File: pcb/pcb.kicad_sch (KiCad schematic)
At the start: 43 parts, among them J1 Conn_01x02_Socket, J2 Conn_01x04_Socket, U1 AP2112K-3.3TRG1, U2 W25Q16JVUXIQ, U3 RP2040, U4 DS4432U+T&amp;R, U5 AD8403ARUZ1-REEL, U6 ADG801BRTZ-REEL7, Y2 Crystal_GND24_Small

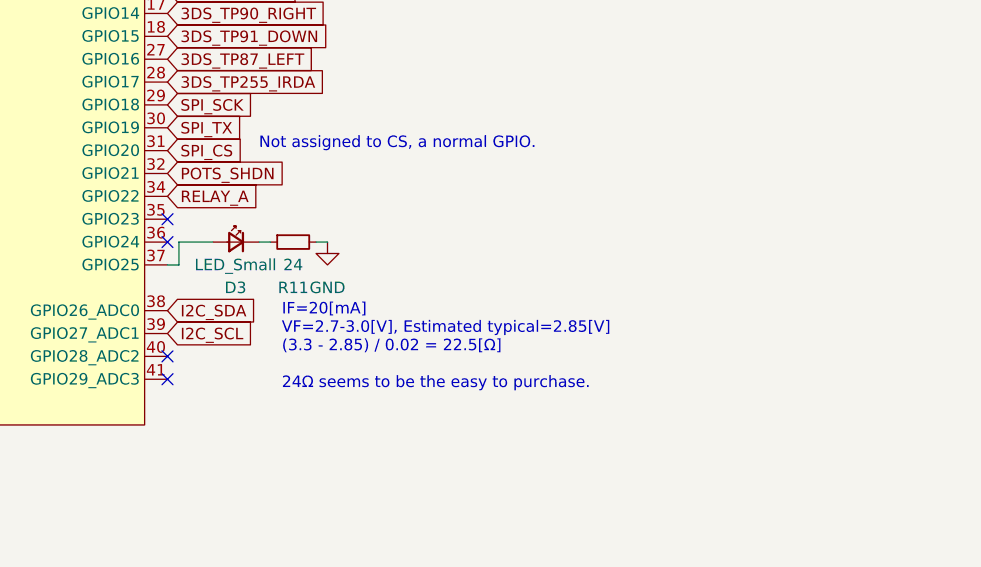
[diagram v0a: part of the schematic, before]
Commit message: Update schematic
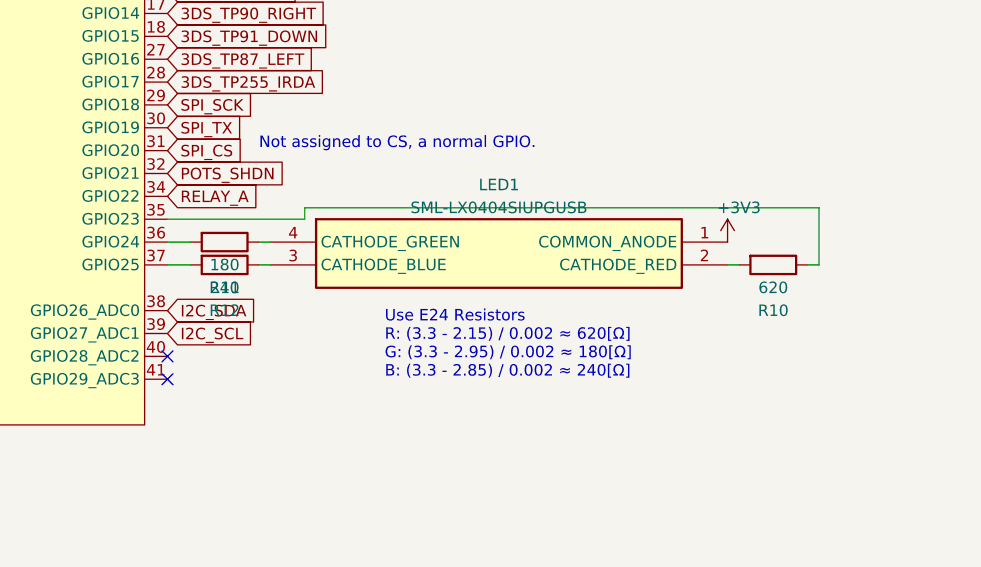
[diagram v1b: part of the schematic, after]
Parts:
- removed D3: LED_Small, LED_SMD:LED_0402_1005Metric, symbol Device:LED_Small
- removed R11: 24, Resistor_SMD:R_0402_1005Metric, symbol Device:R_Small
- added LED1: SML-LX0404SIUPGUSB, SML-LX0404SIUPGUSB, symbol SML-LX0404SIUPGUSB:SML-LX0404SIUPGUSB
- added R10: 620, Resistor_SMD:R_0402_1005Metric, symbol Device:R
- added R11: 180, Resistor_SMD:R_0402_1005Metric, symbol Device:R
- added R12: 240, Resistor_SMD:R_0402_1005Metric, symbol Device:R
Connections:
- net +3V3: now also LED1.1 (COMMON_ANODE)
- net at U3.35 (GPIO23): now also R10.1
- net at U3.36 (GPIO24): now also R11.2
- net at U3.37 (GPIO25): now also R12.2
- new net: LED1.2 (CATHODE_RED), R10.2
- new net: LED1.3 (CATHODE_BLUE), R12.1
- new net: LED1.4 (CATHODE_GREEN), R11.1
- no-connect marks 13 -> 11
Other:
- note added: "Use E24 Resistors R: (3.3 - 2.15) / 0.002 ≈ 620[Ω] G: (3.3 - 2.95) / 0.002 ≈ 180[Ω] B: (3.3 - 2.85) / 0.002 ≈ 240[Ω]"
- note removed: "IF=20[mA] VF=2.7-3.0[V], Estimated typical=2.85[V] (3.3 - 2.85) / 0.02 = 22.5[Ω] 24Ω seems to be the easy to purchase."

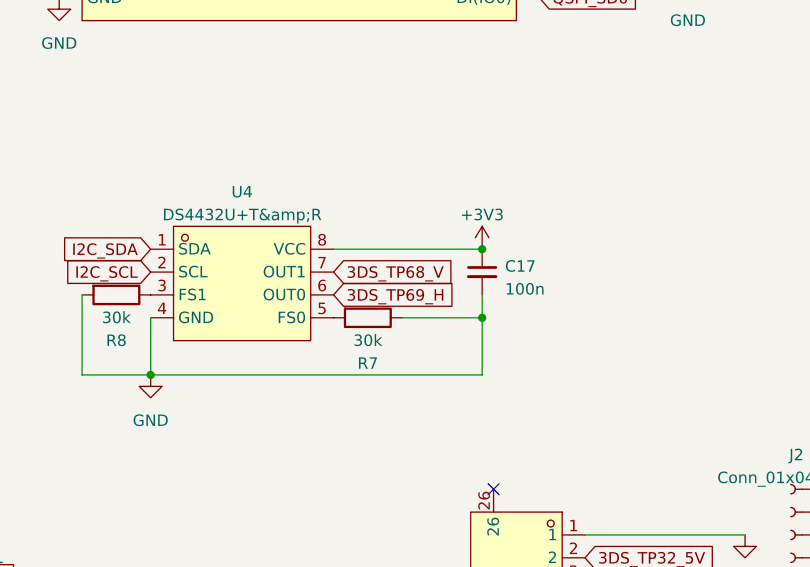
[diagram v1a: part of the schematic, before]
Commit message: Update PCB
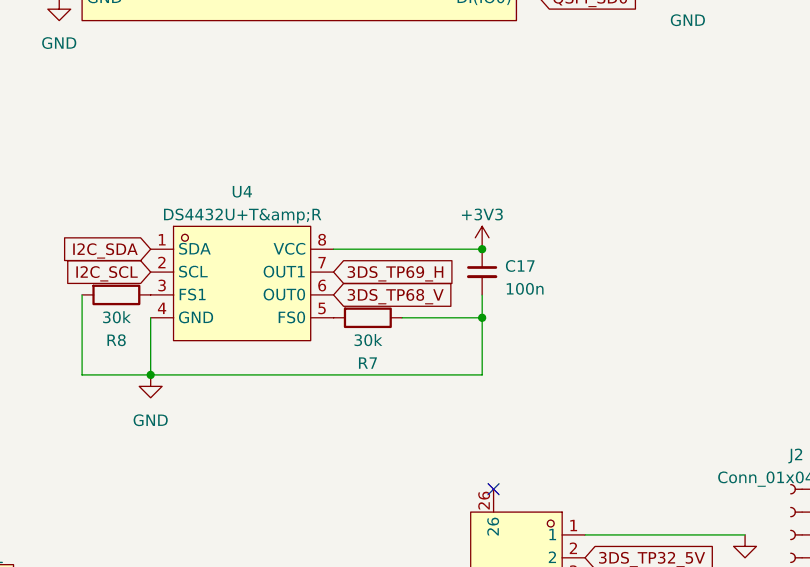
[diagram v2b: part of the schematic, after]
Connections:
- net 3DS_TP68_V: now also U4.6 (OUT0); no longer U4.7 (OUT1)
- net 3DS_TP69_H: now also U4.7 (OUT1); no longer U4.6 (OUT0)

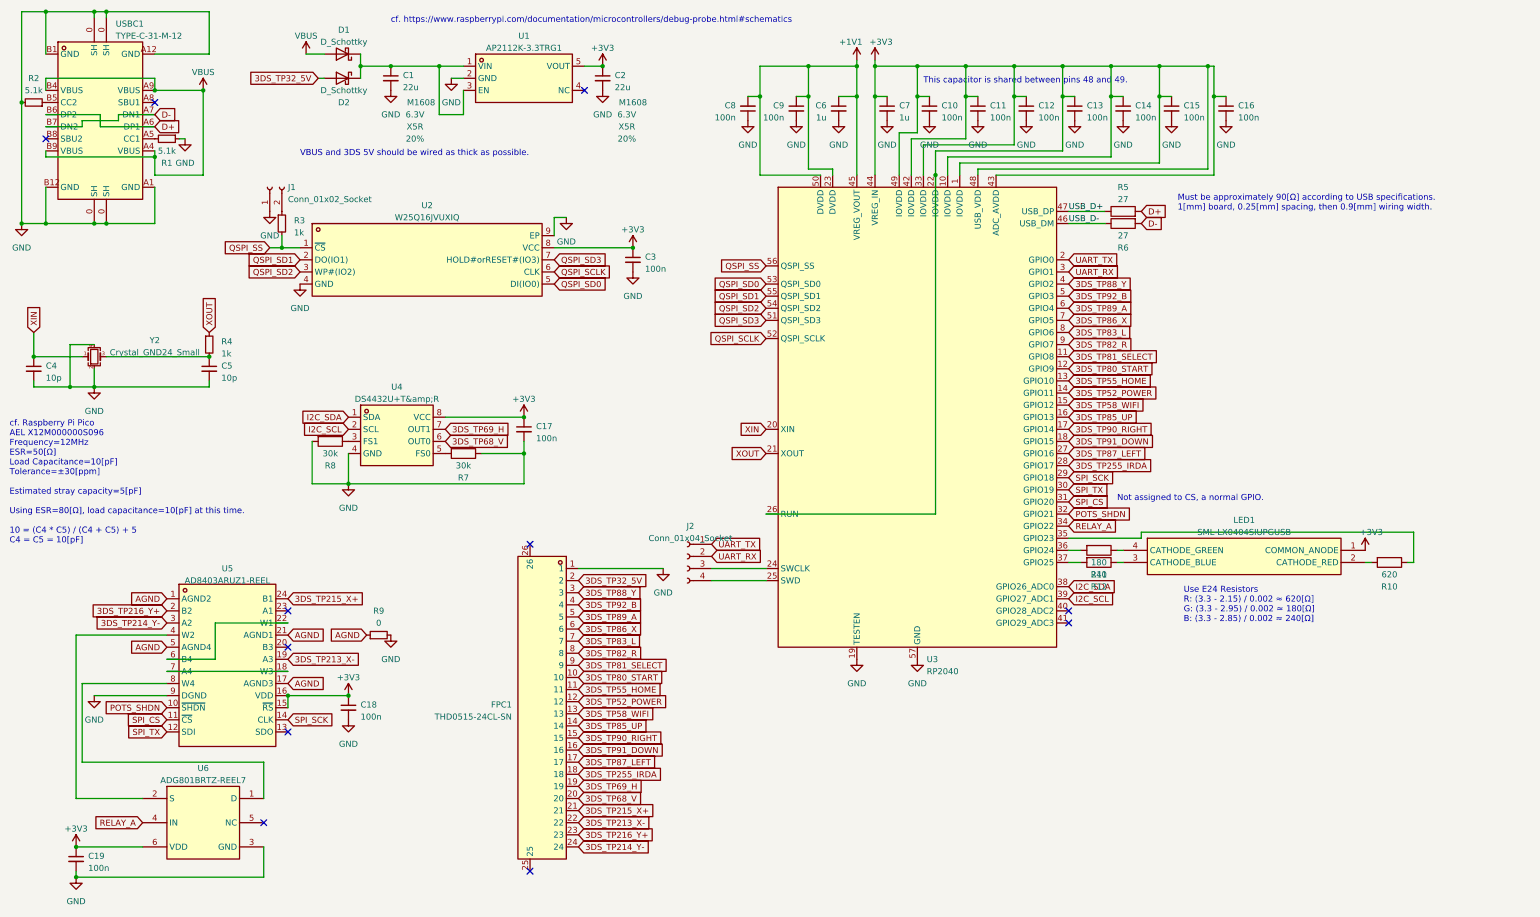
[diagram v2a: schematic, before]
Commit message: Resize
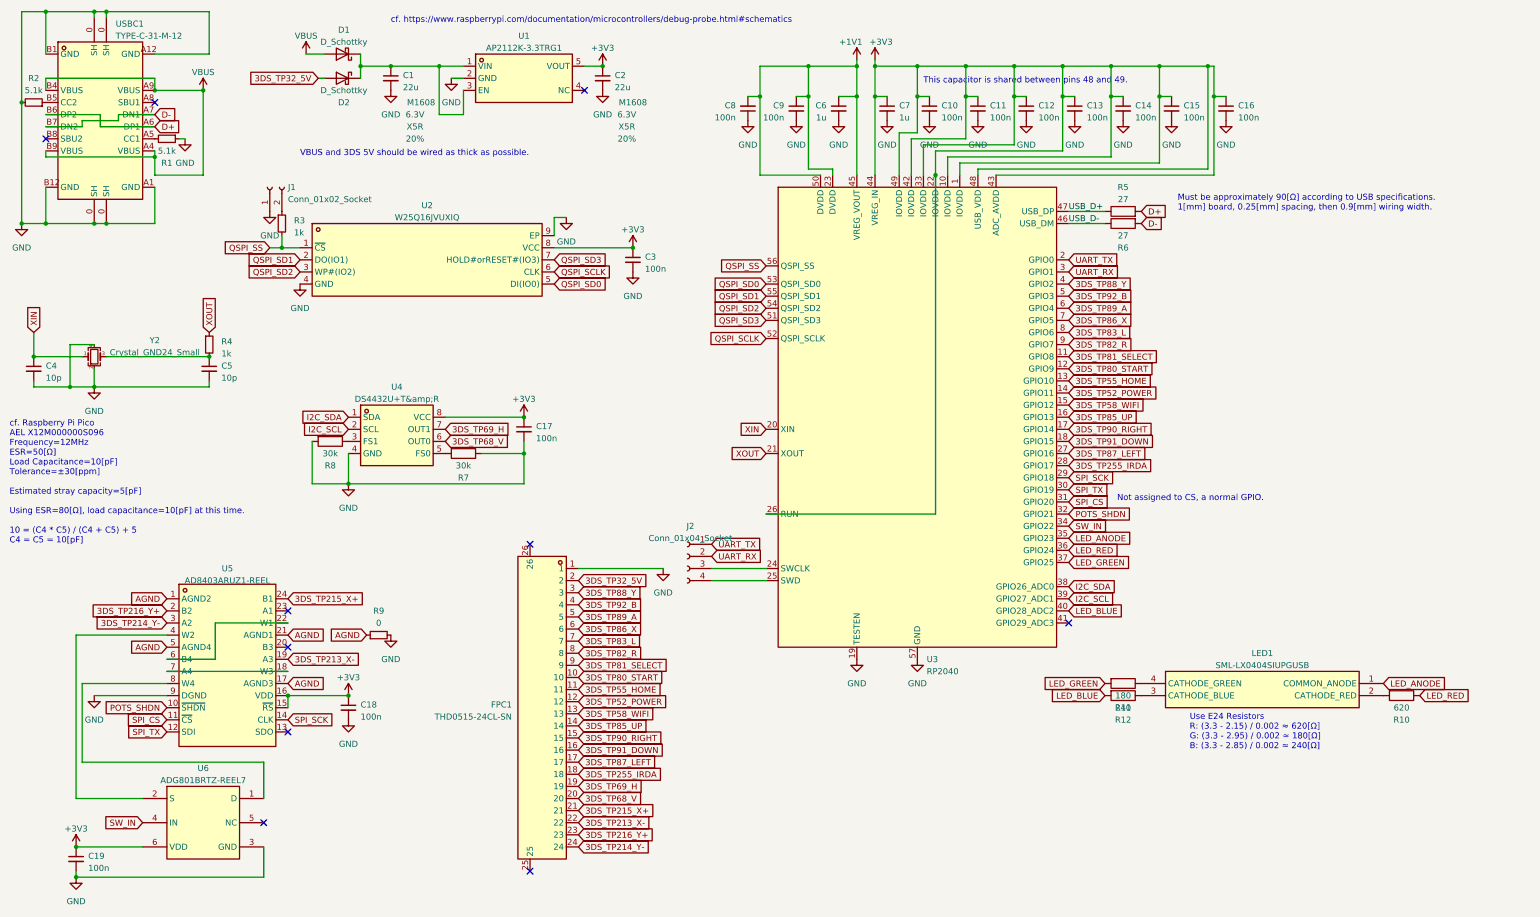
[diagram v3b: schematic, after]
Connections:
- net +3V3: no longer LED1.1 (COMMON_ANODE)
- net LED_ANODE: now reaches U3.35 (GPIO23)
- net LED_ANODE: now also LED1.1 (COMMON_ANODE); no longer R10.1
- net LED_GREEN: now reaches R11.2
- net LED_GREEN: now also U3.37 (GPIO25); no longer U3.36 (GPIO24)
- net LED_BLUE: now reaches R12.2
- net LED_BLUE: now also U3.40 (GPIO28_ADC2); no longer U3.37 (GPIO25)
- net RELAY_A renamed SW_IN
- new net LED_RED: R10.1, U3.36 (GPIO24)
- no-connect marks 11 -> 10
